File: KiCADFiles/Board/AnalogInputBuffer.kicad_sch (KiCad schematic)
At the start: 19 parts, among them U15 OPA1655D, U16 OPA1655D

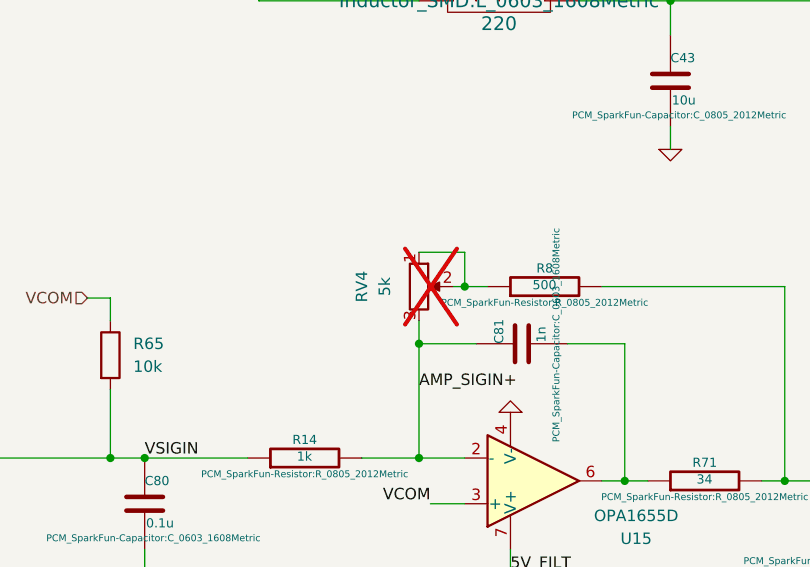
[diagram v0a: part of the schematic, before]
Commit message: improved layout further
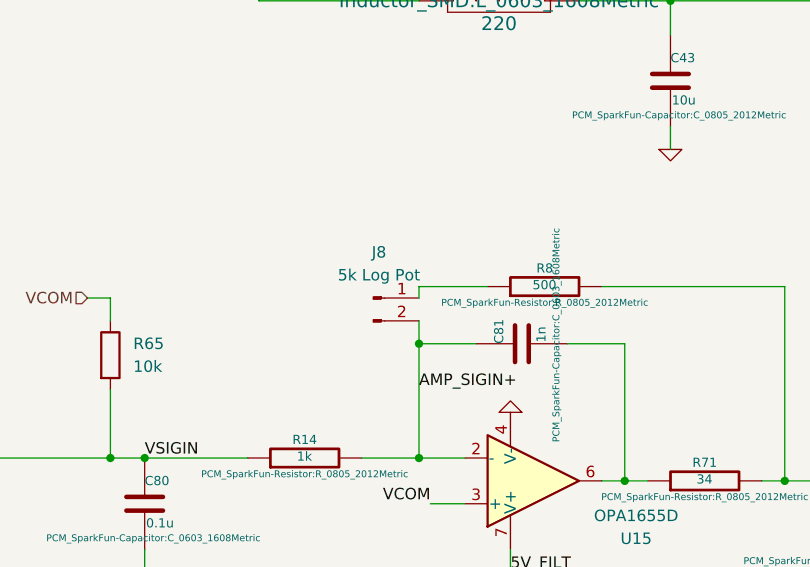
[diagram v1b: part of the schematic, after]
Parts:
- removed RV4: 5k, Potentiometer_THT:Potentiometer_Alps_RK163_Single_Horizontal, symbol Device:R_Potentiometer
- added J8: 5k Log Pot, Connector_PinHeader_2.54mm:PinHeader_1x02_P2.54mm_Vertical, symbol Connector:Conn_01x02_Pin
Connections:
- net AMP_SIGIN+: now also J8.2 (Pin_2)
- net at R8.1: now also J8.1 (Pin_1)
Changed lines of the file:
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@@
-	)
-	(junction
-		(at 129.54 59.69)
-		(diameter 0)
-		(color 0 0 0 0)
 	)
 	(junction
@@
 	(wire
 		(pts
+			(xy 124.46 59.69) (xy 132.08 59.69)
+		)
+		(stroke
+			(width 0)
+			(type default)
+		)
+	)
+	(wire
+		(pts
 			(xy 124.46 78.74) (xy 129.54 78.74)
 		)
@@
 	(wire
 		(pts
-			(xy 124.46 55.88) (xy 129.54 55.88)
-		)
-		(stroke
-			(width 0)
-			(type default)
-		)
-	)
-	(wire
-		(pts
 			(xy 90.17 71.12) (xy 90.17 78.74)
 		)
@@
 	(wire
 		(pts
-			(xy 129.54 59.69) (xy 132.08 59.69)
-		)
-		(stroke
-			(width 0)
-			(type default)
-		)
-	)
-	(wire
-		(pts
 			(xy 158.75 115.57) (xy 158.75 138.43)
 		)
@@
 	(wire
 		(pts
-			(xy 128.27 59.69) (xy 129.54 59.69)
-		)
-		(stroke
-			(width 0)
-			(type default)
-		)
-	)
-	(wire
-		(pts
 			(xy 140.97 66.04) (xy 147.32 66.04)
 		)
@@
 	(wire
 		(pts
+			(xy 124.46 60.96) (xy 124.46 59.69)
+		)
+		(stroke
+			(width 0)
+			(type default)
+		)
+	)
+	(wire
+		(pts
 			(xy 144.78 138.43) (xy 146.05 138.43)
 		)
@@
 		(pts
 			(xy 125.73 140.97) (xy 129.54 140.97)
-		)
-		(stroke
-			(width 0)
-			(type default)
-		)
-	)
-	(wire
-		(pts
-			(xy 129.54 55.88) (xy 129.54 59.69)
 		)
 		(stroke
@@
 	)
 	(symbol
-		(lib_id "Device:R_Potentiometer")
-		(at 124.46 59.69 0)
-		(unit 1)
-		(exclude_from_sim no)
-		(in_bom yes)
-		(on_board yes)
-		(dnp yes)
-		(property "Reference" "RV4"
-			(at 118.11 59.69 90)
-			(effects
-				(font
-					(size 1.27 1.27)
-				)
-			)
-		)
-		(property "Value" "5k"
-			(at 120.65 59.69 90)
-			(effects
-				(font
-					(size 1.27 1.27)
-				)
-			)
-		)
-		(property "Footprint" "Potentiometer_THT:Potentiometer_Alps_RK163_Single_Horizontal"
-			(at 124.46 59.69 0)
-			(effects
-				(font
-					(size 1.27 1.27)
-				)
-				(hide yes)
-			)
-		)
-		(property "Datasheet" "~"
-			(at 124.46 59.69 0)
-			(effects
-				(font
-					(size 1.27 1.27)
-				)
-				(hide yes)
-			)
-		)
-		(property "Description" "Potentiometer"
-			(at 124.46 59.69 0)
-			(effects
-				(font
-					(size 1.27 1.27)
-				)
-				(hide yes)
-			)
-		)
-		(property "MPN" "RV16AF-10-15K-C5K-3LA "
-			(at 124.46 59.69 0)
-			(effects
-				(font
-					(size 1.27 1.27)
-				)
-				(hide yes)
-			)
-		)
-		(property "Tol" ""
-			(at 124.46 59.69 0)
-			(effects
-				(font
-					(size 1.27 1.27)
-				)
-				(hide yes)
-			)
-		)
-		(pin "3"
-		)
-		(pin "2"
-		)
-		(pin "1"
-		)
-		(instances
-			(project "SuperAudioBoard"
-				(path "/01f65e03-4e05-4001-87b4-b3e88e4198ab/00000000-0000-0000-0000-00005438c479/00000000-0000-0000-0000-0000544f05bf"
-					(reference "RV4")
-					(unit 1)
-				)
-				(path "/01f65e03-4e05-4001-87b4-b3e88e4198ab/00000000-0000-0000-0000-00005438c479/00000000-0000-0000-0000-00005456b8dd"
-					(reference "RV5")
-					(unit 1)
-				)
-			)
-		)
-	)
-	(symbol
 		(lib_name "C_16")
 		(lib_id "SuperAudioBoard-rescue:C")
@@
 					(unit 1)
 				)
+			)
+		)
+	)
+	(symbol
+		(lib_id "Connector:Conn_01x02_Pin")
+		(at 119.38 60.96 0)
+		(unit 1)
+		(exclude_from_sim no)
+		(in_bom yes)
+		(on_board yes)
+		(dnp no)
+		(fields_autoplaced yes)
+		(property "Reference" "J8"
+			(at 120.015 55.88 0)
+			(effects
+				(font
+					(size 1.27 1.27)
+				)
+			)
+		)
+		(property "Value" "5k Log Pot"
+			(at 120.015 58.42 0)
+			(effects
+				(font
+					(size 1.27 1.27)
+				)
+			)
+		)
+		(property "Footprint" "Connector_PinHeader_2.54mm:PinHeader_1x02_P2.54mm_Vertical"
+			(at 119.38 60.96 0)
+			(effects
+				(font
+					(size 1.27 1.27)
+				)
+				(hide yes)
+			)
+		)
+		(property "Datasheet" "~"
+			(at 119.38 60.96 0)
+			(effects
+				(font
+					(size 1.27 1.27)
+				)
+				(hide yes)
+			)
+		)
+		(property "Description" "Generic connector, single row, 01x02, script generated"
+			(at 119.38 60.96 0)
+			(effects
+				(font
+					(size 1.27 1.27)
+				)
+				(hide yes)
+			)
+		)
+		(property "MPN" "RV16AF-10-15K-C5K-3LA "
+			(at 119.38 60.96 0)
+			(effects
+				(font
+					(size 1.27 1.27)
+				)
+				(hide yes)
+			)
+		)
+		(pin "2"
+		)
+		(pin "1"
+		)
+		(instances
+			(project ""
+				(path "/01f65e03-4e05-4001-87b4-b3e88e4198ab/00000000-0000-0000-0000-00005438c479/00000000-0000-0000-0000-0000544f05bf"
+					(reference "J8")
+					(unit 1)
+				)
+				(path "/01f65e03-4e05-4001-87b4-b3e88e4198ab/00000000-0000-0000-0000-00005438c479/00000000-0000-0000-0000-00005456b8dd"
+					(reference "J9")
+					(unit 1)
+				)
